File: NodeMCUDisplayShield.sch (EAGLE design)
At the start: 2 parts

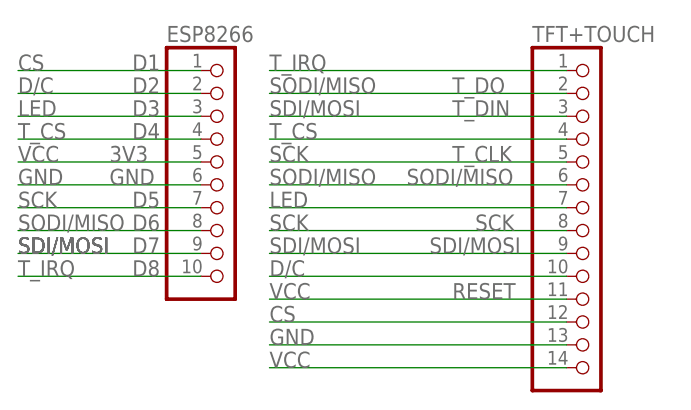
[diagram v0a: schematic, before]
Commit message: Single-sided version
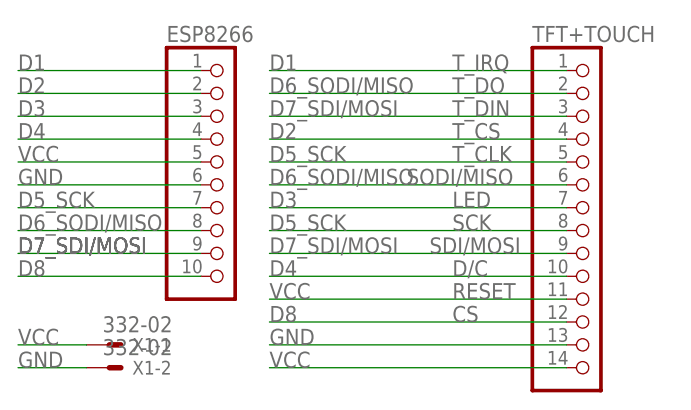
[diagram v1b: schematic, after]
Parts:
- added X1: 332-02, con-garry:332-02
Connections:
- net LED renamed D3
- net SCK renamed D5_SCK
- net SDI/MOSI renamed D7_SDI/MOSI
- net SODI/MISO renamed D6_SODI/MISO
- removed net CS: ESP8266.1, TFT+TOUCH.12
- removed net D/C: ESP8266.2, TFT+TOUCH.10
- removed net T_CS: ESP8266.4, TFT+TOUCH.4
- removed net T_IRQ: ESP8266.10, TFT+TOUCH.1
- new net D1: ESP8266.1, TFT+TOUCH.1
- new net D2: ESP8266.2, TFT+TOUCH.4
- new net D4: ESP8266.4, TFT+TOUCH.10
- new net D8: ESP8266.10, TFT+TOUCH.12
- net GND: now also X1-2.S
- net VCC: now also X1-1.S
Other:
- note added: "CS"
- note added: "D/C"
- note added: "LED"
- note added: "T_CS"
- note added: "T_IRQ"
- note removed: "3V3"
- note removed: "D1"
- note removed: "D2"
- note removed: "D3"
- note removed: "D4"
- note removed: "D5"
- note removed: "D6"
- note removed: "D7"
- note removed: "D8"
- note removed: "GND"
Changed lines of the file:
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@@
 <?xml version="1.0" encoding="utf-8"?>
 <!DOCTYPE eagle SYSTEM "eagle.dtd">
-<eagle version="8.1.0">
+<eagle version="8.3.1">
 <drawing>
 <settings>
 <setting alwaysvectorfont="no"/>
+<setting keepoldvectorfont="yes"/>
 <setting verticaltext="up"/>
 </settings>
@@
 <part name="TFT+TOUCH" library="pinhead" deviceset="PINHD-1X14" device=""/>
 <part name="ESP8266" library="pinhead" deviceset="PINHD-1X10" device=""/>
+<part name="X1" library="con-garry" library_urn="urn:adsk.eagle:library:147" deviceset="332-02" device="" package3d_urn="urn:adsk.eagle:package:6810/1"/>
 </parts>
 <sheets>
 <sheet>
 <plain>
-<text x="22.86" y="68.58" size="1.778" layer="95">D1</text>
-<text x="22.86" y="66.04" size="1.778" layer="95">D2</text>
-<text x="22.86" y="63.5" size="1.778" layer="95">D3</text>
-<text x="22.86" y="60.96" size="1.778" layer="95">D4</text>
-<text x="20.32" y="58.42" size="1.778" layer="95">3V3</text>
-<text x="20.32" y="55.88" size="1.778" layer="95">GND</text>
-<text x="22.86" y="53.34" size="1.778" layer="95">D5</text>
-<text x="22.86" y="50.8" size="1.778" layer="95">D6</text>
-<text x="22.86" y="48.26" size="1.778" layer="95">D7</text>
-<text x="22.86" y="45.72" size="1.778" layer="95">D8</text>
 <text x="58.42" y="58.42" size="1.778" layer="95">T_CLK</text>
 <text x="58.42" y="66.04" size="1.778" layer="95">T_DO</text>
 <text x="58.42" y="63.5" size="1.778" layer="95">T_DIN</text>
-<text x="60.96" y="50.8" size="1.778" layer="95">SCK</text>
+<text x="58.42" y="50.8" size="1.778" layer="95">SCK</text>
 <text x="55.88" y="48.26" size="1.778" layer="95">SDI/MOSI</text>
 <text x="58.42" y="43.18" size="1.778" layer="95">RESET</text>
 <text x="53.34" y="55.88" size="1.778" layer="95">SODI/MISO</text>
+<text x="58.42" y="68.58" size="1.778" layer="95">T_IRQ</text>
+<text x="58.42" y="60.96" size="1.778" layer="95">T_CS</text>
+<text x="58.42" y="53.34" size="1.778" layer="95">LED</text>
+<text x="58.42" y="45.72" size="1.778" layer="95">D/C</text>
+<text x="58.42" y="40.64" size="1.778" layer="95">CS</text>
 </plain>
 <instances>
 <instance part="TFT+TOUCH" gate="A" x="73.66" y="53.34"/>
 <instance part="ESP8266" gate="A" x="33.02" y="58.42"/>
+<instance part="X1" gate="-1" x="20.32" y="38.1"/>
+<instance part="X1" gate="-2" x="20.32" y="35.56"/>
 </instances>
 <busses>
 </busses>
 <nets>
-<net name="T_IRQ" class="0">
-<segment>
-<pinref part="TFT+TOUCH" gate="A" pin="1"/>
-<wire x1="71.12" y1="68.58" x2="38.1" y2="68.58" width="0.1524" layer="91"/>
-<label x="38.1" y="68.58" size="1.778" layer="95"/>
-</segment>
+<net name="D8" class="0">
 <segment>
 <pinref part="ESP8266" gate="A" pin="10"/>
@@
 <label x="10.16" y="45.72" size="1.778" layer="95"/>
 </segment>
-</net>
-<net name="T_CS" class="0">
-<segment>
-<pinref part="TFT+TOUCH" gate="A" pin="4"/>
-<wire x1="71.12" y1="60.96" x2="38.1" y2="60.96" width="0.1524" layer="91"/>
-<label x="38.1" y="60.96" size="1.778" layer="95"/>
-</segment>
+<segment>
+<pinref part="TFT+TOUCH" gate="A" pin="12"/>
+<wire x1="71.12" y1="40.64" x2="38.1" y2="40.64" width="0.1524" layer="91"/>
+<label x="38.1" y="40.64" size="1.778" layer="95"/>
+</segment>
+</net>
+<net name="D4" class="0">
 <segment>
 <pinref part="ESP8266" gate="A" pin="4"/>
@@
 <label x="10.16" y="60.96" size="1.778" layer="95"/>
 </segment>
-</net>
-<net name="SODI/MISO" class="0">
+<segment>
+<pinref part="TFT+TOUCH" gate="A" pin="10"/>
+<wire x1="71.12" y1="45.72" x2="38.1" y2="45.72" width="0.1524" layer="91"/>
+<label x="38.1" y="45.72" size="1.778" layer="95"/>
+</segment>
+</net>
+<net name="D6_SODI/MISO" class="0">
 <segment>
 <pinref part="TFT+TOUCH" gate="A" pin="6"/>
@@
 </segment>
 </net>
-<net name="LED" class="1">
+<net name="D3" class="1">
 <segment>
 <pinref part="TFT+TOUCH" gate="A" pin="7"/>
@@
 </segment>
 </net>
-<net name="SCK" class="0">
+<net name="D5_SCK" class="0">
 <segment>
 <pinref part="TFT+TOUCH" gate="A" pin="8"/>
@@
 </segment>
 </net>
-<net name="SDI/MOSI" class="0">
+<net name="D7_SDI/MOSI" class="0">
 <segment>
 <pinref part="TFT+TOUCH" gate="A" pin="9"/>
@@
 </segment>
 </net>
-<net name="D/C" class="0">
-<segment>
-<pinref part="TFT+TOUCH" gate="A" pin="10"/>
-<wire x1="71.12" y1="45.72" x2="38.1" y2="45.72" width="0.1524" layer="91"/>
-<label x="38.1" y="45.72" size="1.778" layer="95"/>
-</segment>
+<net name="D2" class="0">
 <segment>
 <pinref part="ESP8266" gate="A" pin="2"/>
@@
 <label x="10.16" y="66.04" size="1.778" layer="95"/>
 </segment>
-</net>
-<net name="CS" class="0">
-<segment>
-<pinref part="TFT+TOUCH" gate="A" pin="12"/>
-<wire x1="71.12" y1="40.64" x2="38.1" y2="40.64" width="0.1524" layer="91"/>
-<label x="38.1" y="40.64" size="1.778" layer="95"/>
-</segment>
+<segment>
+<pinref part="TFT+TOUCH" gate="A" pin="4"/>
+<wire x1="71.12" y1="60.96" x2="38.1" y2="60.96" width="0.1524" layer="91"/>
+<label x="38.1" y="60.96" size="1.778" layer="95"/>
+</segment>
+</net>
+<net name="D1" class="0">
 <segment>
 <pinref part="ESP8266" gate="A" pin="1"/>
@@
 <label x="10.16" y="68.58" size="1.778" layer="95"/>
 </segment>
+<segment>
+<pinref part="TFT+TOUCH" gate="A" pin="1"/>
+<wire x1="71.12" y1="68.58" x2="38.1" y2="68.58" width="0.1524" layer="91"/>
+<label x="38.1" y="68.58" size="1.778" layer="95"/>
+</segment>
 </net>
 <net name="GND" class="1">
@@
 <label x="10.16" y="55.88" size="1.778" layer="95"/>
 </segment>
+<segment>
+<pinref part="X1" gate="-2" pin="S"/>
+<wire x1="17.78" y1="35.56" x2="10.16" y2="35.56" width="0.1524" layer="91"/>
+<label x="10.16" y="35.56" size="1.778" layer="95"/>
+</segment>
 </net>
 <net name="VCC" class="1">
@@
 <wire x1="71.12" y1="43.18" x2="38.1" y2="43.18" width="0.1524" layer="91"/>
 <label x="38.1" y="43.18" size="1.778" layer="95"/>
+</segment>
+<segment>
+<pinref part="X1" gate="-1" pin="S"/>
+<wire x1="17.78" y1="38.1" x2="10.16" y2="38.1" width="0.1524" layer="91"/>
+<label x="10.16" y="38.1" size="1.778" layer="95"/>
 </segment>
 </net>
@@
 </schematic>
 </drawing>
+<compatibility>
+<note version="8.2" severity="warning">
+Since Version 8.2, EAGLE supports online libraries. The ids
+of those online libraries will not be understood (or retained)
+with this version.
+</note>
+<note version="8.3" severity="warning">
+Since Version 8.3, EAGLE supports URNs for individual library
+assets (packages, symbols, and devices). The URNs of those assets
+will not be understood (or retained) with this version.
+</note>
+<note version="8.3" severity="warning">
+Since Version 8.3, EAGLE supports the association of 3D packages
+with devices in libraries, schematics, and board files. Those 3D
+packages will not be understood (or retained) with this version.
+</note>
+</compatibility>
 </eagle>
